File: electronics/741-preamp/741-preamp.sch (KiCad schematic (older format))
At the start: 14 parts, among them J1 PWR, J2 Audio In, J3 OUT, U1 LM741

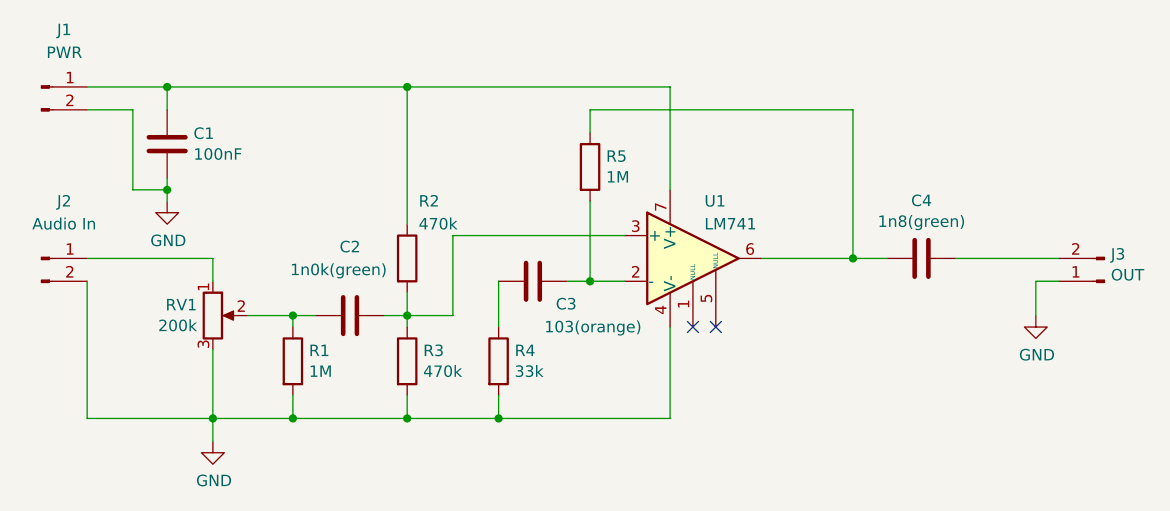
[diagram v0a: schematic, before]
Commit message: PCB
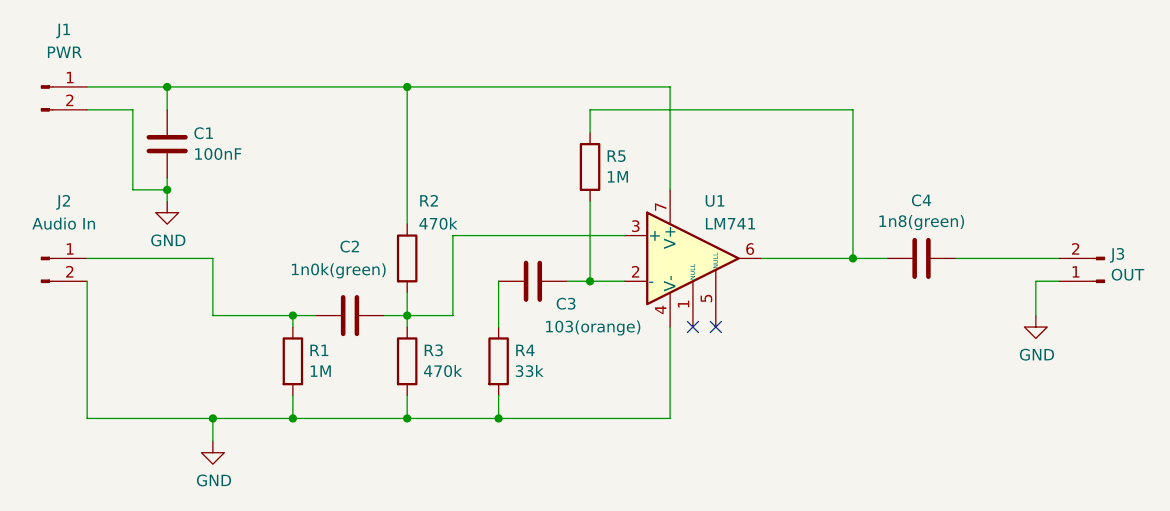
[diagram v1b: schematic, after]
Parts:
- removed RV1: 200k, symbol Device:R_POT
- C1, C2, C3, C4: footprint (none) -> Capacitor_THT:C_Disc_D4.3mm_W1.9mm_P5.00mm
- J1, J2, J3: footprint (none) -> Connector_PinHeader_2.54mm:PinHeader_1x02_P2.54mm_Vertical
- R1, R2, R3, R4, R5: footprint (none) -> Resistor_THT:R_Axial_DIN0204_L3.6mm_D1.6mm_P7.62mm_Horizontal
- U1: footprint (none) -> Package_DIP:DIP-8_W7.62mm
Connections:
- net at J2.1 (Pin_1): now also C2.2, R1.1
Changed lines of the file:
@@
 EESchema Schematic File Version 4
+LIBS:741-preamp-cache
 EELAYER 30 0
 EELAYER END
@@
 $EndDescr
 $Comp
-L Device:R_POT RV1
-U 1 1 5DCDABE7
-P 2450 2050
-F 0 "RV1" H 2381 2096 50  0000 R CNN
-F 1 "200k" H 2381 2005 50  0000 R CNN
-F 2 "" H 2450 2050 50  0001 C CNN
-F 3 "~" H 2450 2050 50  0001 C CNN
-	1    2450 2050
-	1    0    0    -1
-$EndComp
-$Comp
 L Amplifier_Operational:LM741 U1
 U 1 1 5DCDAEE1
@@
 F 0 "U1" H 4600 2050 50  0000 L CNN
 F 1 "LM741" H 4600 1950 50  0000 L CNN
-F 2 "" H 4600 1850 50  0001 C CNN
+F 2 "Package_DIP:DIP-8_W7.62mm" H 4600 1850 50  0001 C CNN
 F 3 "http://www.ti.com/lit/ds/symlink/lm741.pdf" H 4700 1950 50  0001 C CNN
 	1    4550 1800
@@
 F 0 "C1" H 2135 1254 50  0000 R CNN
 F 1 "100nF" H 2135 1345 50  0000 R CNN
-F 2 "" H 2288 1150 50  0001 C CNN
+F 2 "Capacitor_THT:C_Disc_D4.3mm_W1.9mm_P5.00mm" H 2288 1150 50  0001 C CNN
 F 3 "~" H 2250 1300 50  0001 C CNN
 	1    2250 1300
@@
 F 0 "C4" V 5298 1800 50  0000 C CNN
 F 1 "1n8(green)" V 5389 1800 50  0000 C CNN
-F 2 "" H 5588 1650 50  0001 C CNN
+F 2 "Capacitor_THT:C_Disc_D4.3mm_W1.9mm_P5.00mm" H 5588 1650 50  0001 C CNN
 F 3 "~" H 5550 1800 50  0001 C CNN
 	1    5550 1800
@@
 F 0 "C2" V 2750 2050 50  0000 C CNN
 F 1 "1n0k(green)" V 2850 2000 50  0000 C CNN
-F 2 "" H 3088 1900 50  0001 C CNN
+F 2 "Capacitor_THT:C_Disc_D4.3mm_W1.9mm_P5.00mm" H 3088 1900 50  0001 C CNN
 F 3 "~" H 3050 2050 50  0001 C CNN
 	1    3050 2050
@@
 F 0 "R4" H 3770 2296 50  0000 L CNN
 F 1 "33k" H 3770 2205 50  0000 L CNN
-F 2 "" V 3630 2250 50  0001 C CNN
+F 2 "Resistor_THT:R_Axial_DIN0204_L3.6mm_D1.6mm_P7.62mm_Horizontal" V 3630 2250 50  0001 C CNN
 F 3 "~" H 3700 2250 50  0001 C CNN
 	1    3700 2250
@@
 F 0 "R5" H 4170 1446 50  0000 L CNN
 F 1 "1M" H 4170 1355 50  0000 L CNN
-F 2 "" V 4030 1400 50  0001 C CNN
+F 2 "Resistor_THT:R_Axial_DIN0204_L3.6mm_D1.6mm_P7.62mm_Horizontal" V 4030 1400 50  0001 C CNN
 F 3 "~" H 4100 1400 50  0001 C CNN
 	1    4100 1400
@@
 F 0 "R1" H 2870 2296 50  0000 L CNN
 F 1 "1M" H 2870 2205 50  0000 L CNN
-F 2 "" V 2730 2250 50  0001 C CNN
+F 2 "Resistor_THT:R_Axial_DIN0204_L3.6mm_D1.6mm_P7.62mm_Horizontal" V 2730 2250 50  0001 C CNN
 F 3 "~" H 2800 2250 50  0001 C CNN
 	1    2800 2250
@@
 F 0 "R3" H 3370 2296 50  0000 L CNN
 F 1 "470k" H 3370 2205 50  0000 L CNN
-F 2 "" V 3230 2250 50  0001 C CNN
+F 2 "Resistor_THT:R_Axial_DIN0204_L3.6mm_D1.6mm_P7.62mm_Horizontal" V 3230 2250 50  0001 C CNN
 F 3 "~" H 3300 2250 50  0001 C CNN
 	1    3300 2250
@@
 F 0 "R2" H 3350 2050 50  0000 L CNN
 F 1 "470k" H 3350 1950 50  0000 L CNN
-F 2 "" V 3230 1800 50  0001 C CNN
+F 2 "Resistor_THT:R_Axial_DIN0204_L3.6mm_D1.6mm_P7.62mm_Horizontal" V 3230 1800 50  0001 C CNN
 F 3 "~" H 3300 1800 50  0001 C CNN
 	1    3300 1800
@@
 F 0 "J1" H 1800 1300 50  0000 C CNN
 F 1 "PWR" H 1800 1200 50  0000 C CNN
-F 2 "" H 1700 1050 50  0001 C CNN
+F 2 "Connector_PinHeader_2.54mm:PinHeader_1x02_P2.54mm_Vertical" H 1700 1050 50  0001 C CNN
 F 3 "~" H 1700 1050 50  0001 C CNN
 	1    1700 1050
@@
 F 0 "J2" H 1800 2050 50  0000 C CNN
 F 1 "Audio In" H 1800 1950 50  0000 C CNN
-F 2 "" H 1700 1800 50  0001 C CNN
+F 2 "Connector_PinHeader_2.54mm:PinHeader_1x02_P2.54mm_Vertical" H 1700 1800 50  0001 C CNN
 F 3 "~" H 1700 1800 50  0001 C CNN
 	1    1700 1800
@@
 F 0 "J3" H 6322 1782 50  0000 R CNN
 F 1 "OUT" H 6322 1873 50  0000 R CNN
-F 2 "" H 6350 1900 50  0001 C CNN
+F 2 "Connector_PinHeader_2.54mm:PinHeader_1x02_P2.54mm_Vertical" H 6350 1900 50  0001 C CNN
 F 3 "~" H 6350 1900 50  0001 C CNN
 	1    6350 1900
@@
 Wire Wire Line
 	1900 1800 2450 1800
-Wire Wire Line
-	2450 1800 2450 1900
 $Comp
 L power:GND #PWR02
@@
 $EndComp
 Wire Wire Line
-	2600 2050 2800 2050
-Wire Wire Line
 	2800 2050 2800 2100
 Wire Wire Line
@@
 Wire Wire Line
 	1900 1900 1900 2500
-Wire Wire Line
-	2450 2200 2450 2500
 Connection ~ 2450 2500
 Wire Wire Line
@@
 F 0 "C3" V 3950 2000 50  0000 L CNN
 F 1 "103(orange)" V 4050 1950 50  0000 L CNN
-F 2 "" H 3888 1750 50  0001 C CNN
+F 2 "Capacitor_THT:C_Disc_D4.3mm_W1.9mm_P5.00mm" H 3888 1750 50  0001 C CNN
 F 3 "~" H 3850 1900 50  0001 C CNN
 	1    3850 1900
@@
 Wire Wire Line
 	3200 2050 3300 2050
+Wire Wire Line
+	2450 1800 2450 2050
+Wire Wire Line
+	2450 2050 2800 2050
 $EndSCHEMATC

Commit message: PCB with connectors
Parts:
- J1, J2, J3: footprint Connector_PinHeader_2.54mm:PinHeader_1x02_P2.54mm_Vertical -> Connector_Phoenix_MC_HighVoltage:PhoenixContact_MCV_1,5_2-G-5.08_1x02_P5.08mm_Vertical
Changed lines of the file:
@@
 F 0 "J1" H 1800 1300 50  0000 C CNN
 F 1 "PWR" H 1800 1200 50  0000 C CNN
-F 2 "Connector_PinHeader_2.54mm:PinHeader_1x02_P2.54mm_Vertical" H 1700 1050 50  0001 C CNN
+F 2 "Connector_Phoenix_MC_HighVoltage:PhoenixContact_MCV_1,5_2-G-5.08_1x02_P5.08mm_Vertical" H 1700 1050 50  0001 C CNN
 F 3 "~" H 1700 1050 50  0001 C CNN
 	1    1700 1050
@@
 F 0 "J2" H 1800 2050 50  0000 C CNN
 F 1 "Audio In" H 1800 1950 50  0000 C CNN
-F 2 "Connector_PinHeader_2.54mm:PinHeader_1x02_P2.54mm_Vertical" H 1700 1800 50  0001 C CNN
+F 2 "Connector_Phoenix_MC_HighVoltage:PhoenixContact_MCV_1,5_2-G-5.08_1x02_P5.08mm_Vertical" H 1700 1800 50  0001 C CNN
 F 3 "~" H 1700 1800 50  0001 C CNN
 	1    1700 1800
@@
 F 0 "J3" H 6322 1782 50  0000 R CNN
 F 1 "OUT" H 6322 1873 50  0000 R CNN
-F 2 "Connector_PinHeader_2.54mm:PinHeader_1x02_P2.54mm_Vertical" H 6350 1900 50  0001 C CNN
+F 2 "Connector_Phoenix_MC_HighVoltage:PhoenixContact_MCV_1,5_2-G-5.08_1x02_P5.08mm_Vertical" H 6350 1900 50  0001 C CNN
 F 3 "~" H 6350 1900 50  0001 C CNN
 	1    6350 1900
